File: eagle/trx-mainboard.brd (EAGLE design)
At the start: 97.6 x 84.5 mm, 38 parts, among them J1 629722000214, J2 DF12NB(3.0)-10DP-0.5V, P1 S2B-PH-SM4-TB, Q1 BSS84, U2 BQ2407X

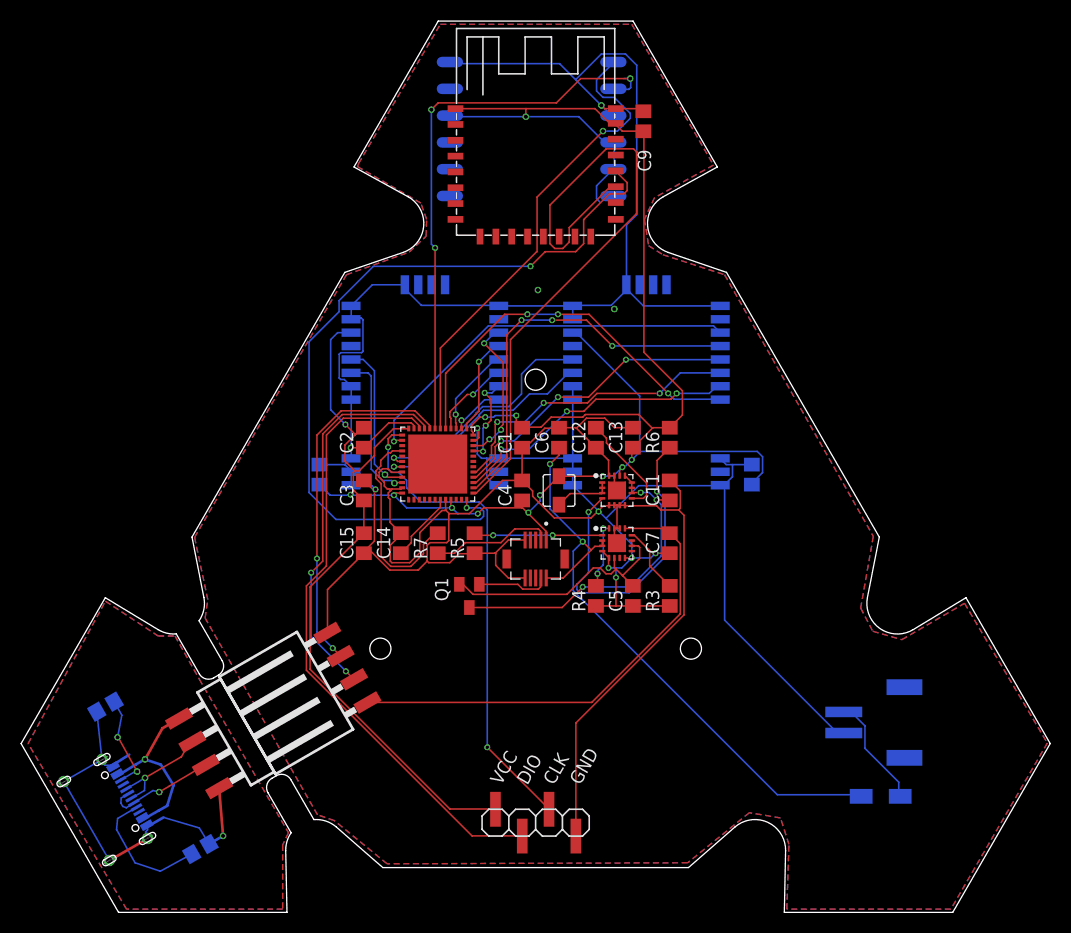
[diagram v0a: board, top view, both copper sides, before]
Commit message: Added new layout and gerber files
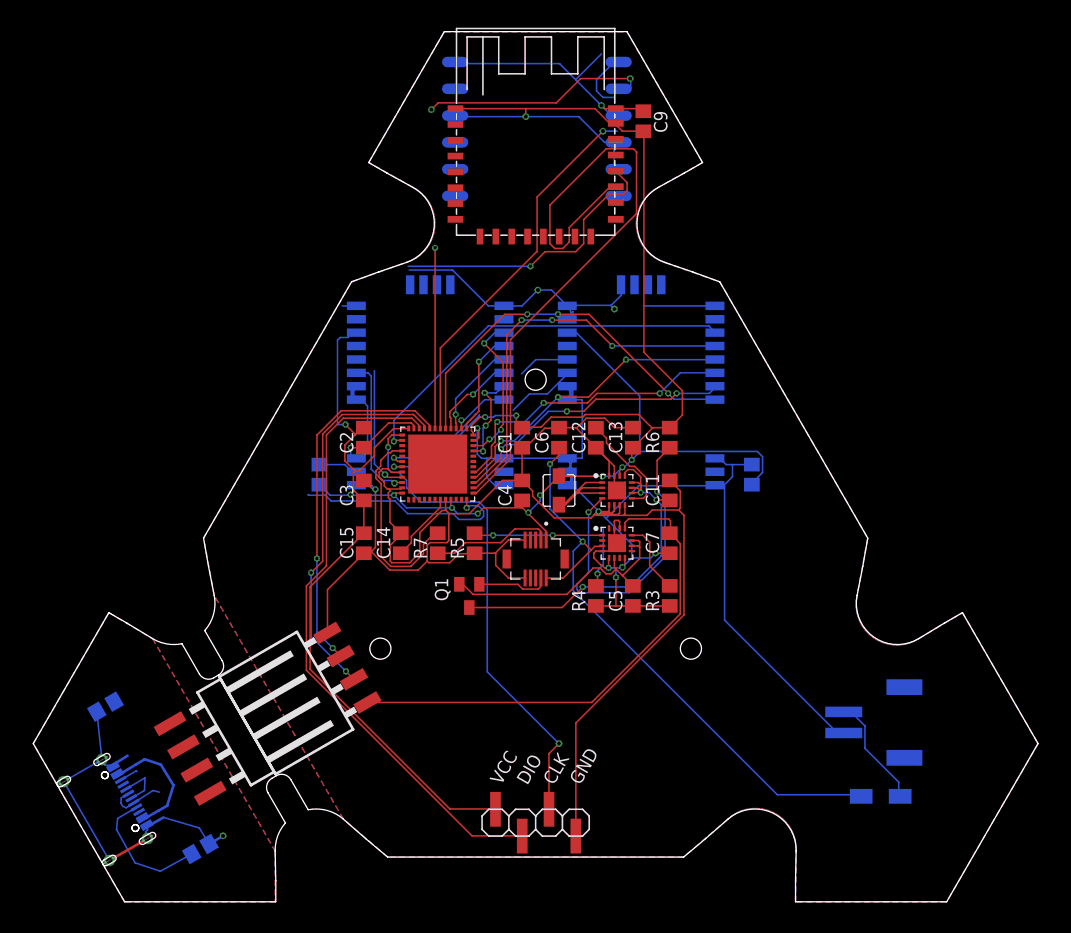
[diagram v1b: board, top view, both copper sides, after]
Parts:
- removed U$6, U$9: E32-X00M20S, ebyte:E32-X00M20S
- added LORA1, LORA2: E32-X00M20S, ebyte:E32-X00M20S
- C11: value 100nF -> 10uF
- C12: value 100nF -> 3.3nF
- R4: value 3k -> 1.8k
- R5: value 3k -> 10k
- R6: value 3k -> 100k
- moved U$1 0.50 mm to (48.9, 74.3)
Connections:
- net +3V3: now also LORA1.9, LORA2.9; no longer U$6.9, U$9.9
- net GND: now also LORA1.1, LORA1.10, LORA1.11, LORA1.12, LORA1.16, LORA1.2, LORA1.24, LORA1.26, LORA1.3, LORA1.4, LORA1.5, LORA2.1, LORA2.10, LORA2.11, LORA2.12, LORA2.16, LORA2.2, LORA2.24, LORA2.26, LORA2.3, LORA2.4, LORA2.5; no longer U$6.1, U$6.10, U$6.11, U$6.12, U$6.16, U$6.2, U$6.24, U$6.26, U$6.3, U$6.4, U$6.5, U$9.1, U$9.10, U$9.11, U$9.12, U$9.16, U$9.2, U$9.24, U$9.26, U$9.3, U$9.4, U$9.5
- net LORA1_D0: now also LORA1.18; no longer U$9.18
- net LORA1_MISO: now also LORA1.20; no longer U$9.20
- net LORA1_MOSI: now also LORA1.21; no longer U$9.21
- net LORA1_RST: now also LORA1.19; no longer U$9.19
- net LORA1_RXEN: now also LORA1.6; no longer U$9.6
- net LORA1_SCK: now also LORA1.22; no longer U$9.22
- net LORA1_SSEL: now also LORA1.23; no longer U$9.23
- net LORA1_TXEN: now also LORA1.7; no longer U$9.7
- net LORA2_D0: now also LORA2.18; no longer U$6.18
- net LORA2_MISO: now also LORA2.20; no longer U$6.20
- net LORA2_MOSI: now also LORA2.21; no longer U$6.21
- net LORA2_RST: now also LORA2.19; no longer U$6.19
- net LORA2_RXEN: now also LORA2.6; no longer U$6.6
- net LORA2_SCK: now also LORA2.22; no longer U$6.22
- net LORA2_SSEL: now also LORA2.23; no longer U$6.23
- net LORA2_TXEN: now also LORA2.7; no longer U$6.7
- net USB_GND: now also U$3.4; no longer U$3.1
- net USB_V: now also U$3.1; no longer U$3.4
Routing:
- net BT_RX: track 75.4 -> 48.3 mm
- net GPS_TX: track 53.7 -> 39.3 mm
- net GND: track 389.4 -> 376.0 mm
- net N$6: track 5.56 -> 13.3 mm
- net LORA1_TXEN: track 22.9 -> 15.4 mm
- net N$2: track 9.26 -> 1.80 mm, vias 2 -> 0
- net USB_D+: track 11.4 -> 4.76 mm, vias 1 -> 0
- net USB_GND: track 41.5 -> 35.6 mm
- net USB_V: track 17.6 -> 12.3 mm, vias 1 -> 0
- net USB_D-: track 10.8 -> 5.64 mm, vias 1 -> 0
- net V+: track 31.6 -> 36.1 mm
- net GPS_RX: track 45.6 -> 41.7 mm
- net LORA1_RXEN: track 21.5 -> 17.7 mm
- net +3V3: track 239.2 -> 235.9 mm
- net VUSB: track 45.6 -> 48.2 mm
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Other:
- board size 97.6 x 84.5 mm -> 95.3 x 82.5 mm
- board text added: "LORA1"
- board text added: "LORA2"
